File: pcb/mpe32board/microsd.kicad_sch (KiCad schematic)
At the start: 6 parts, among them J44 Micro_SD_Card

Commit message: layout stuff
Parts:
- J44: footprint (none) -> Connector_Card:microSD_HC_Molex_47219-2001
- R95, R96, R97, R98, R99: footprint (none) -> Resistor_SMD:R_0603_1608Metric
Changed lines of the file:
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@@
 			)
 		)
-		(property "Footprint" ""
+		(property "Footprint" "Resistor_SMD:R_0603_1608Metric"
 			(at 134.62 68.58 0)
 			(effects
@@
 			)
 		)
-		(property "Footprint" ""
+		(property "Footprint" "Resistor_SMD:R_0603_1608Metric"
 			(at 119.38 68.58 0)
 			(effects
@@
 			)
 		)
-		(property "Footprint" ""
+		(property "Footprint" "Connector_Card:microSD_HC_Molex_47219-2001"
 			(at 204.47 76.2 0)
 			(effects
@@
 			)
 		)
-		(property "Footprint" ""
+		(property "Footprint" "Resistor_SMD:R_0603_1608Metric"
 			(at 111.76 68.58 0)
 			(effects
@@
 			)
 		)
-		(property "Footprint" ""
+		(property "Footprint" "Resistor_SMD:R_0603_1608Metric"
 			(at 127 68.58 0)
 			(effects
@@
 			)
 		)
-		(property "Footprint" ""
+		(property "Footprint" "Resistor_SMD:R_0603_1608Metric"
 			(at 142.24 68.58 0)
 			(effects

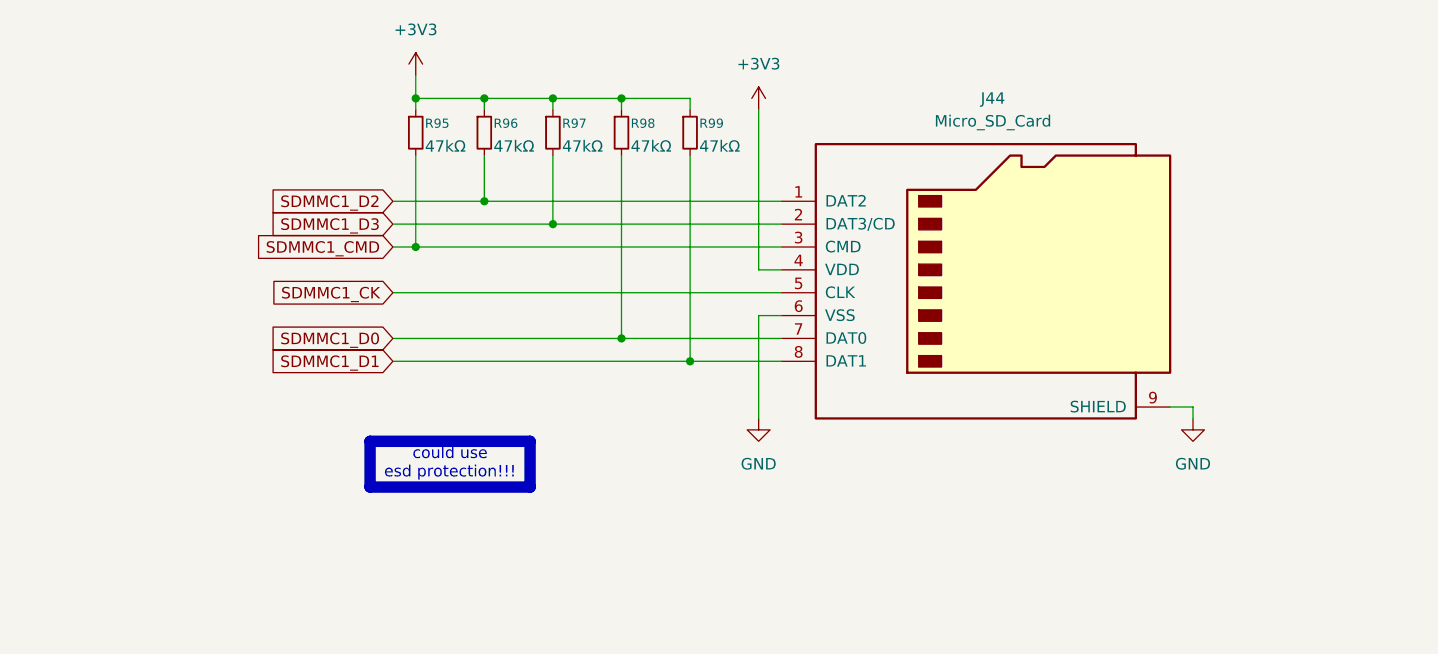
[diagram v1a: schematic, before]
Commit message: board layout stuff
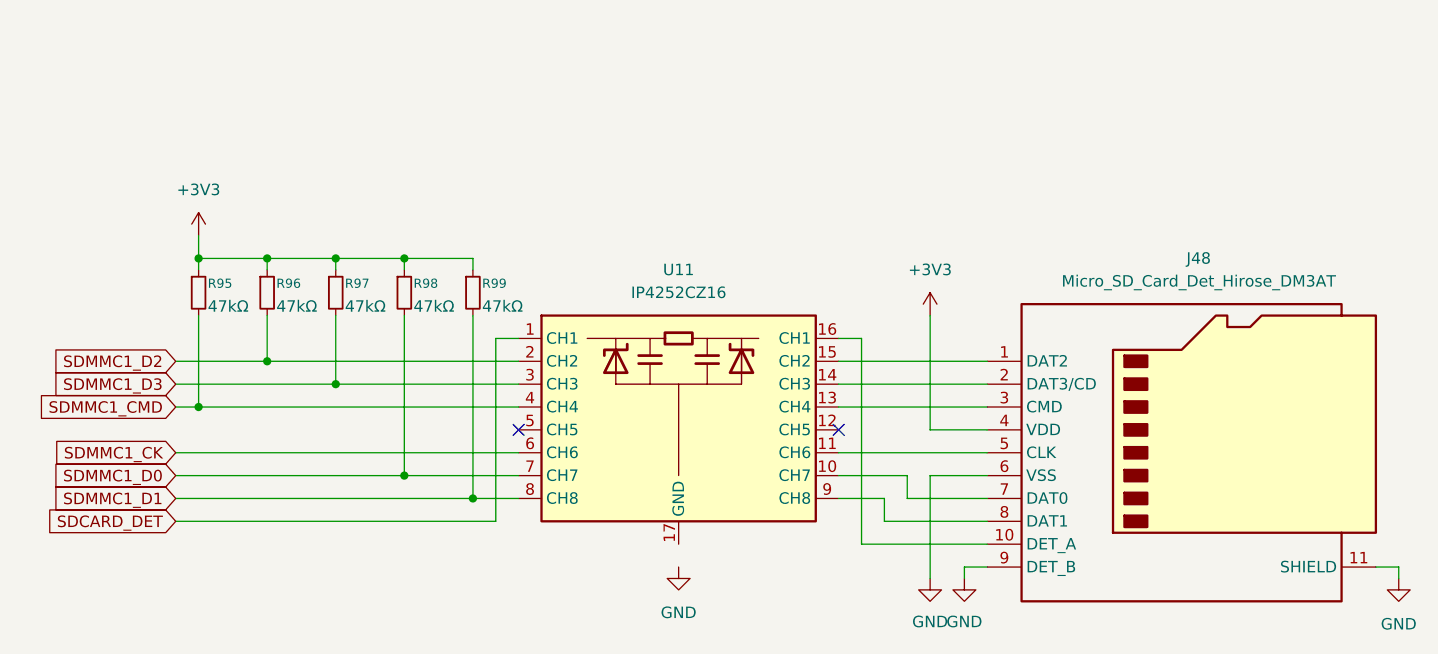
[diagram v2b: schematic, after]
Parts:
- removed J44: Micro_SD_Card, Connector_Card:microSD_HC_Molex_47219-2001, symbol Connector:Micro_SD_Card
- added J48: Micro_SD_Card_Det_Hirose_DM3AT, Connector_Card:microSD_HC_Hirose_DM3D-SF, symbol Connector:Micro_SD_Card_Det_Hirose_DM3AT
- added U11: IP4252CZ16, Package_SON:Nexperia_HUSON-16_USON-16-1EP_1.35x3.3mm_P0.4mm_EP0.4x2.8mm, symbol Power_Protection:IP4252CZ16
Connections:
- net +3V3: now also J48.4 (VDD)
- net GND: now also J48.11 (SHIELD), J48.6 (VSS), J48.9 (DET_B)
- net SDMMC1_CK: now also U11.6 (CH6)
- net SDMMC1_CMD: now also U11.4 (CH4)
- net SDMMC1_D0: now also U11.7 (CH7)
- net SDMMC1_D1: now also U11.8 (CH8)
- net SDMMC1_D2: now also U11.2 (CH2)
- net SDMMC1_D3: now also U11.3 (CH3)
- new net: J48.7 (DAT0), U11.10 (CH7)
- new net: J48.5 (CLK), U11.11 (CH6)
- new net: J48.3 (CMD), U11.13 (CH4)
- new net: J48.2 (DAT3/CD), U11.14 (CH3)
- new net: J48.1 (DAT2), U11.15 (CH2)
- new net: J48.10 (DET_A), U11.16 (CH1)
- new net: J48.8 (DAT1), U11.9 (CH8)
- new net SDCARD_DET: U11.1 (CH1)
- no-connect marks 0 -> 2
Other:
- note removed: "could use esd protection!!!"
- moved on the sheet: R95, R96, R97, R98, R99
